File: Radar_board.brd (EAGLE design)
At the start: 97.8 x 53.4 mm, 31 parts, among them IC1 555, IC2 TPS7A0533PDBVR, J1 AUDIO_JACK_3.5MM_PTH, Q2 MMBT2222ALT1, Q3 MMBT2222ALT1, Q4 MMBT2222ALT1, U1 MAX2750AUA+, U2 NE5532DR

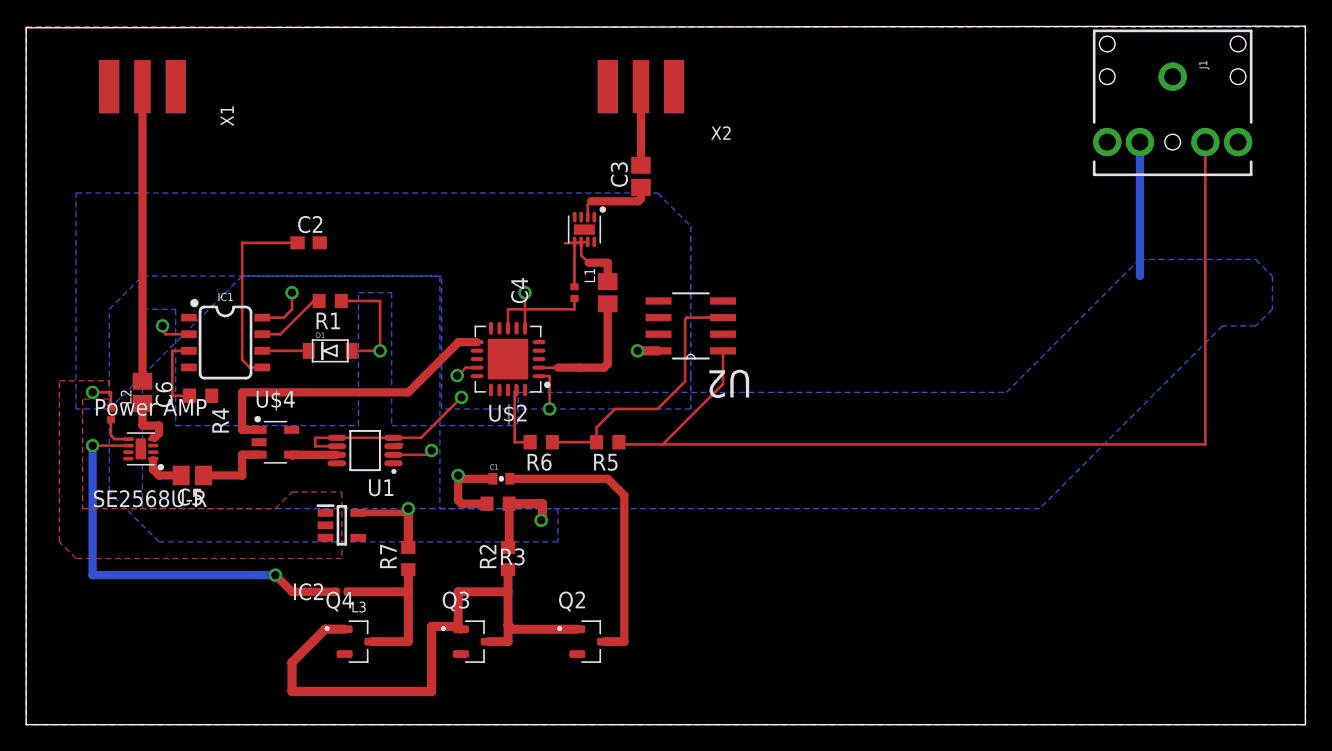
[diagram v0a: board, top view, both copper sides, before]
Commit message: Add files via upload
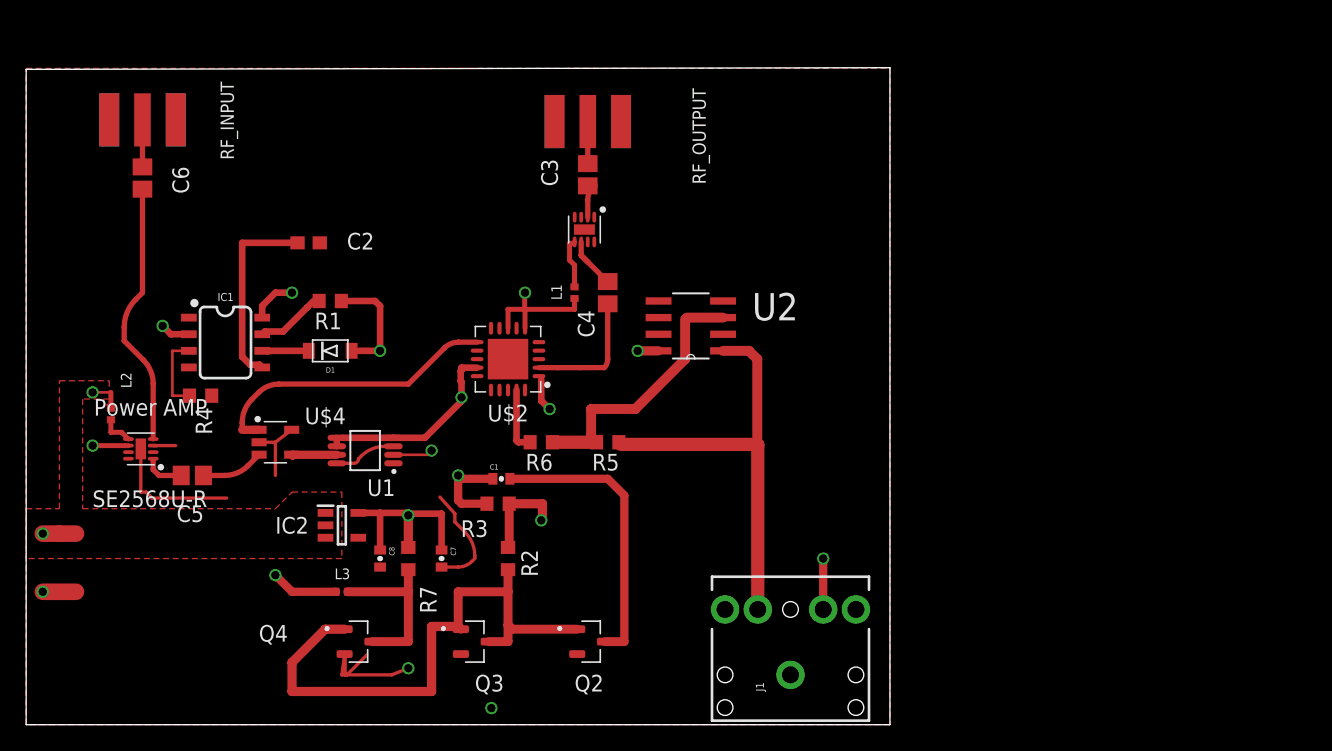
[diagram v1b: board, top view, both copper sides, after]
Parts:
- removed X1, X2: (no value), adafruit:SMA_EDGELAUNCH
- added C7: 0.1uF, SparkFun-Retired:0402-CAP
- added C8: 1uF, SparkFun-Retired:0402-CAP
- added RF_INPUT, RF_OUTPUT: (no value), adafruit:SMA_EDGELAUNCH
- moved J1 54.3 mm to (58.4, 3.81), turned to 90 degrees
- moved C6 16.4 mm to (8.89, 41.8)
- moved C3 4.07 mm to (42.9, 42.0)
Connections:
- removed net 0: C2.2, IC1.1, IC1.4, IC2.2, Q2.2, Q3.2, Q4.2, R4.1, U$1.7, U$2.10, U$2.12, U$2.13, U$2.15, U$2.16, U$2.17, U$2.18, U$2.20, U$2.21, U$2.3, U$2.4, U$2.5, U$2.9, U$3.2, U$3.3, U$3.9, U$4.2, U$4.5, U1.3, U1.8, U2.2, U2.4, U2.5, U2.6, X1.GND@1, X1.GND@2, X1.GND@3, X1.GND@4, X2.GND@1, X2.GND@2, X2.GND@3, X2.GND@4
- new net GND: C2.2, C7.2, C8.2, IC1.1, IC1.4, IC2.2, Q2.2, Q3.2, Q4.2, R4.1, RF_INPUT.GND@1, RF_INPUT.GND@2, RF_INPUT.GND@3, RF_INPUT.GND@4, RF_OUTPUT.GND@1, RF_OUTPUT.GND@2, RF_OUTPUT.GND@3, RF_OUTPUT.GND@4, U$1.7, U$2.10, U$2.12, U$2.13, U$2.15, U$2.16, U$2.17, U$2.18, U$2.20, U$2.21, U$2.3, U$2.4, U$2.5, U$2.9, U$3.2, U$3.3, U$3.9, U$4.2, U$4.5, U1.3, U1.8, U2.2, U2.4, U2.5, U2.6
- net N$10: now also RF_OUTPUT.P; no longer X2.P
- net N$14: now also RF_INPUT.P; no longer X1.P
- net VCC3V: now also C7.1, C8.1
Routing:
- net GND: track 0.00 -> 51.0 mm, vias 0 -> 3
- net N$15: track 77.1 -> 32.8 mm
- net N$14: track 22.5 -> 3.59 mm
- net N$12: track 4.13 -> 20.5 mm
- net VCC3V: track 18.0 -> 25.6 mm
- net N$10: track 6.01 -> 1.56 mm
- net N$8: track 6.06 -> 2.94 mm
- net 0: track 3.03 -> 0.00 mm
- net VCC6V: track 34.5 -> 32.0 mm, vias 6 -> 5
- net N$17: track 0.00 -> 2.54 mm, vias 0 -> 1
- net TRIOUT: track 31.9 -> 29.8 mm, vias 4 -> 5
- net LO_SPLIT: track 23.7 -> 22.6 mm
- net PA_IN: track 5.84 -> 4.75 mm
- added copper zone on layer 1, net GND
- added copper zone on layer 15, net GND
- added copper zone on layer 15, net TRIOUT
- added copper zone on layer 15, net VCC3V
- added copper zone on layer 15, net VCC6V
- removed copper zone on layer 1, net 0
- removed copper zone on layer 16, net GND
- removed copper zone on layer 16, net TRIOUT
- removed copper zone on layer 16, net VCC3V
- removed copper zone on layer 16, net VCC6V
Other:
- board size 97.8 x 53.4 mm -> 66 x 50.2 mm
